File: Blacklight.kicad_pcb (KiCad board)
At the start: 2 copper layers, 54.6 x 52.7 mm, 39 parts, among them J1 Conn_01x06_Female, J2 Barrel_Jack_Switch, Q1 BC547, Q2 BC547, Q3 BC547, Q4 BC547

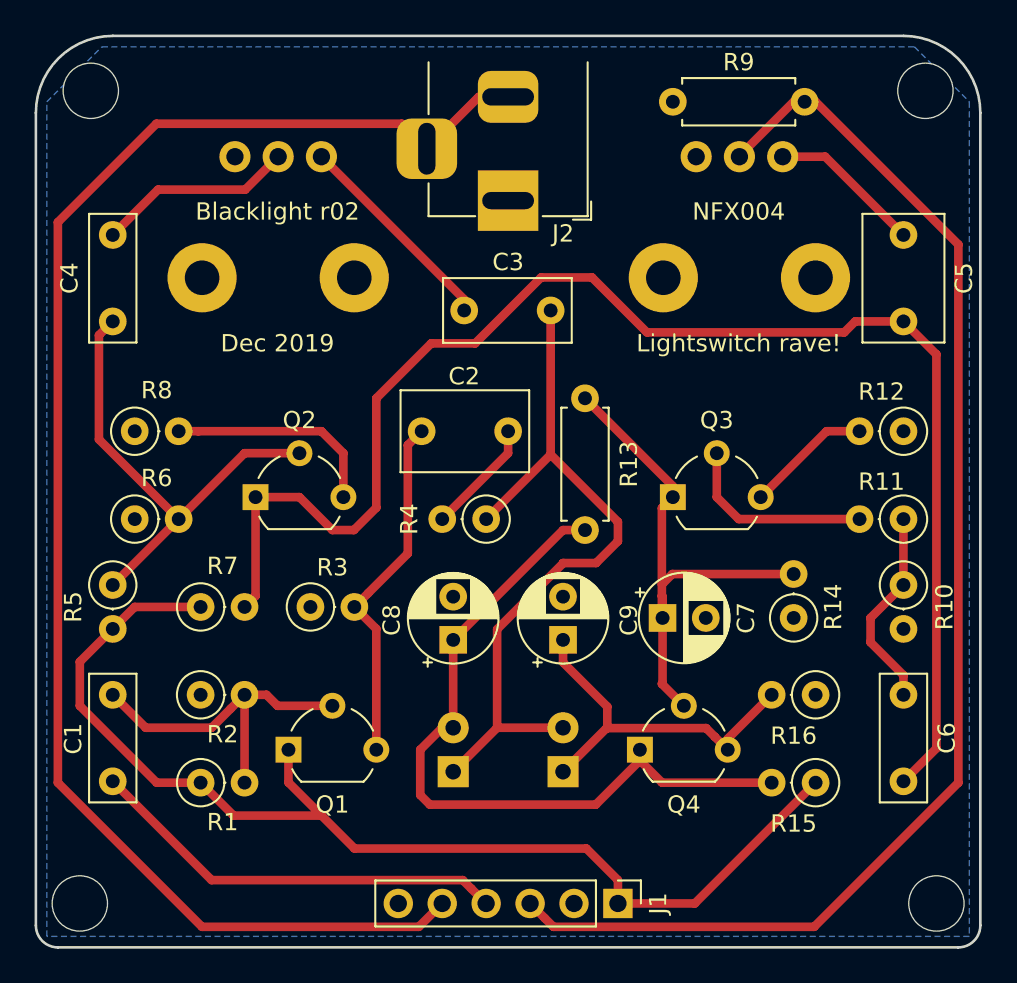
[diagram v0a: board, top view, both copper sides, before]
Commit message: Migrate to KiCAD 6
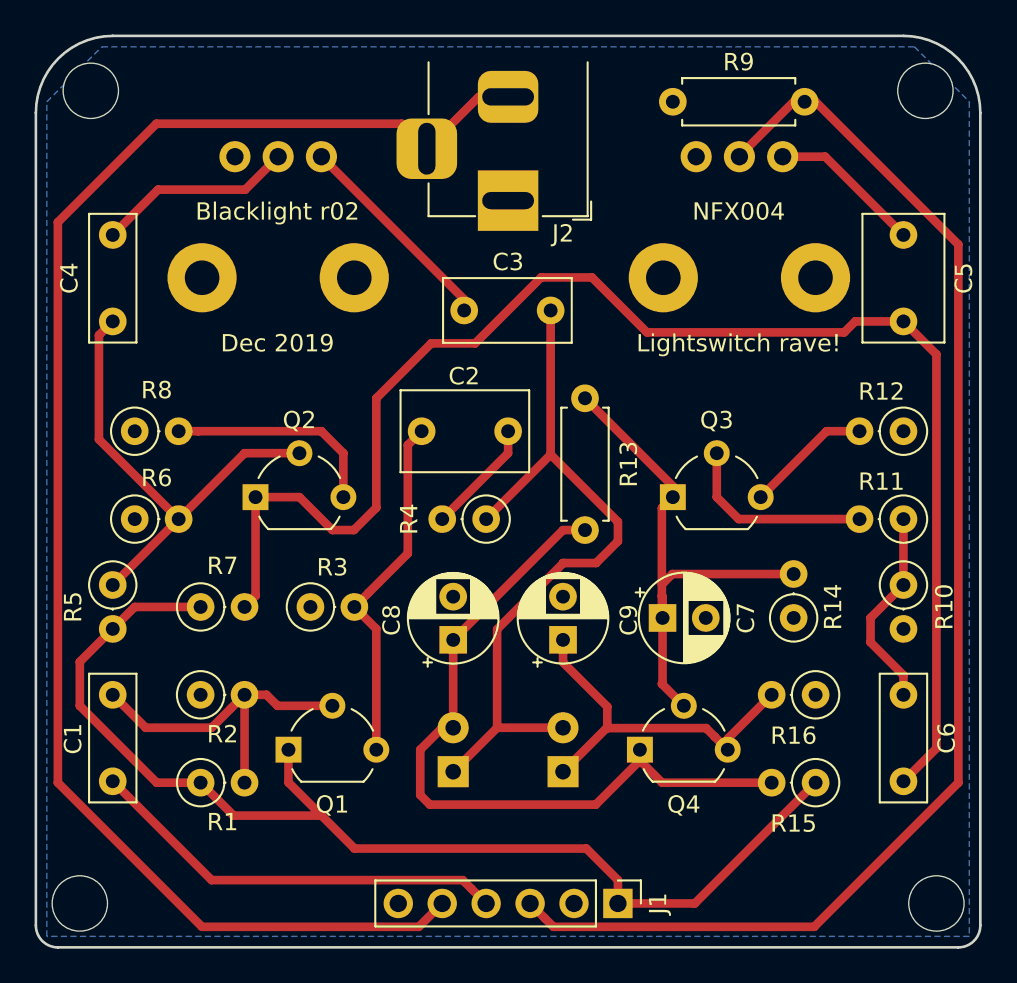
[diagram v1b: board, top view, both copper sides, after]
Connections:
- J1 pad 2: Net-(J1-Pad2) -> unconnected-(J1-Pad2)
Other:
- net class Default removed
